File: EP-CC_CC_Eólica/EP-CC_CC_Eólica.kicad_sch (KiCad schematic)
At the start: 19 parts, among them J1 Screw_Terminal_01x03, J2 Screw_Terminal_01x02, Q1 IKW40N120H3, U1 LA100-P, U2 LV25-P

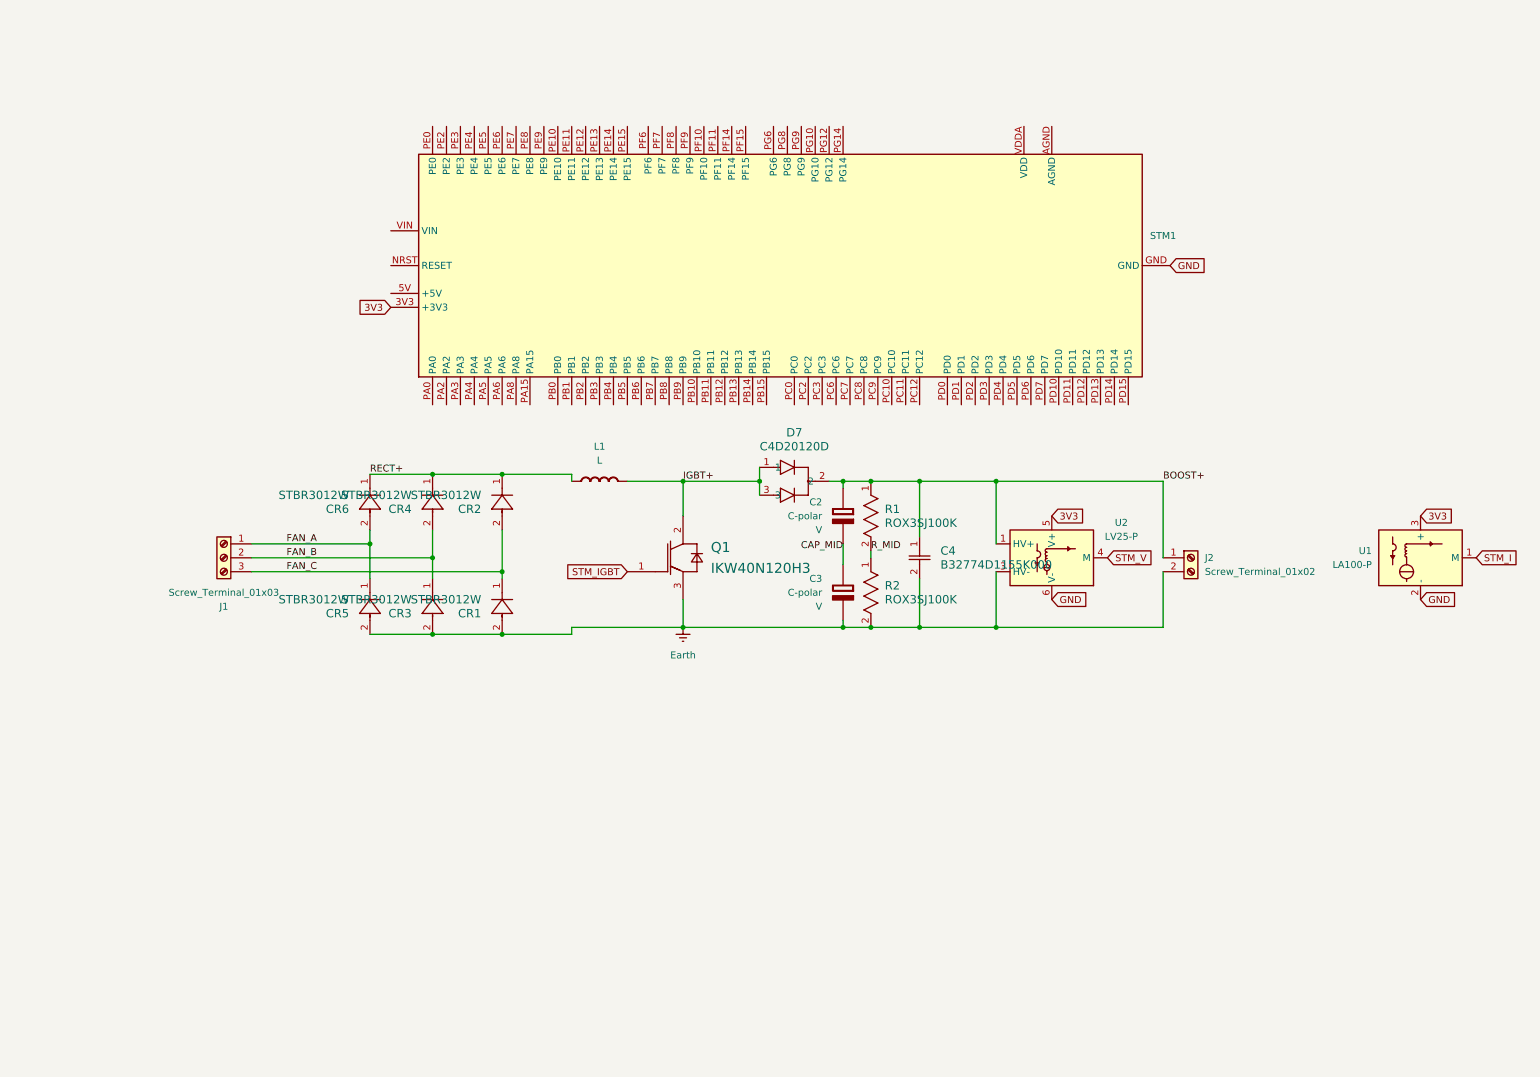
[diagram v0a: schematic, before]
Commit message: 26/10/19
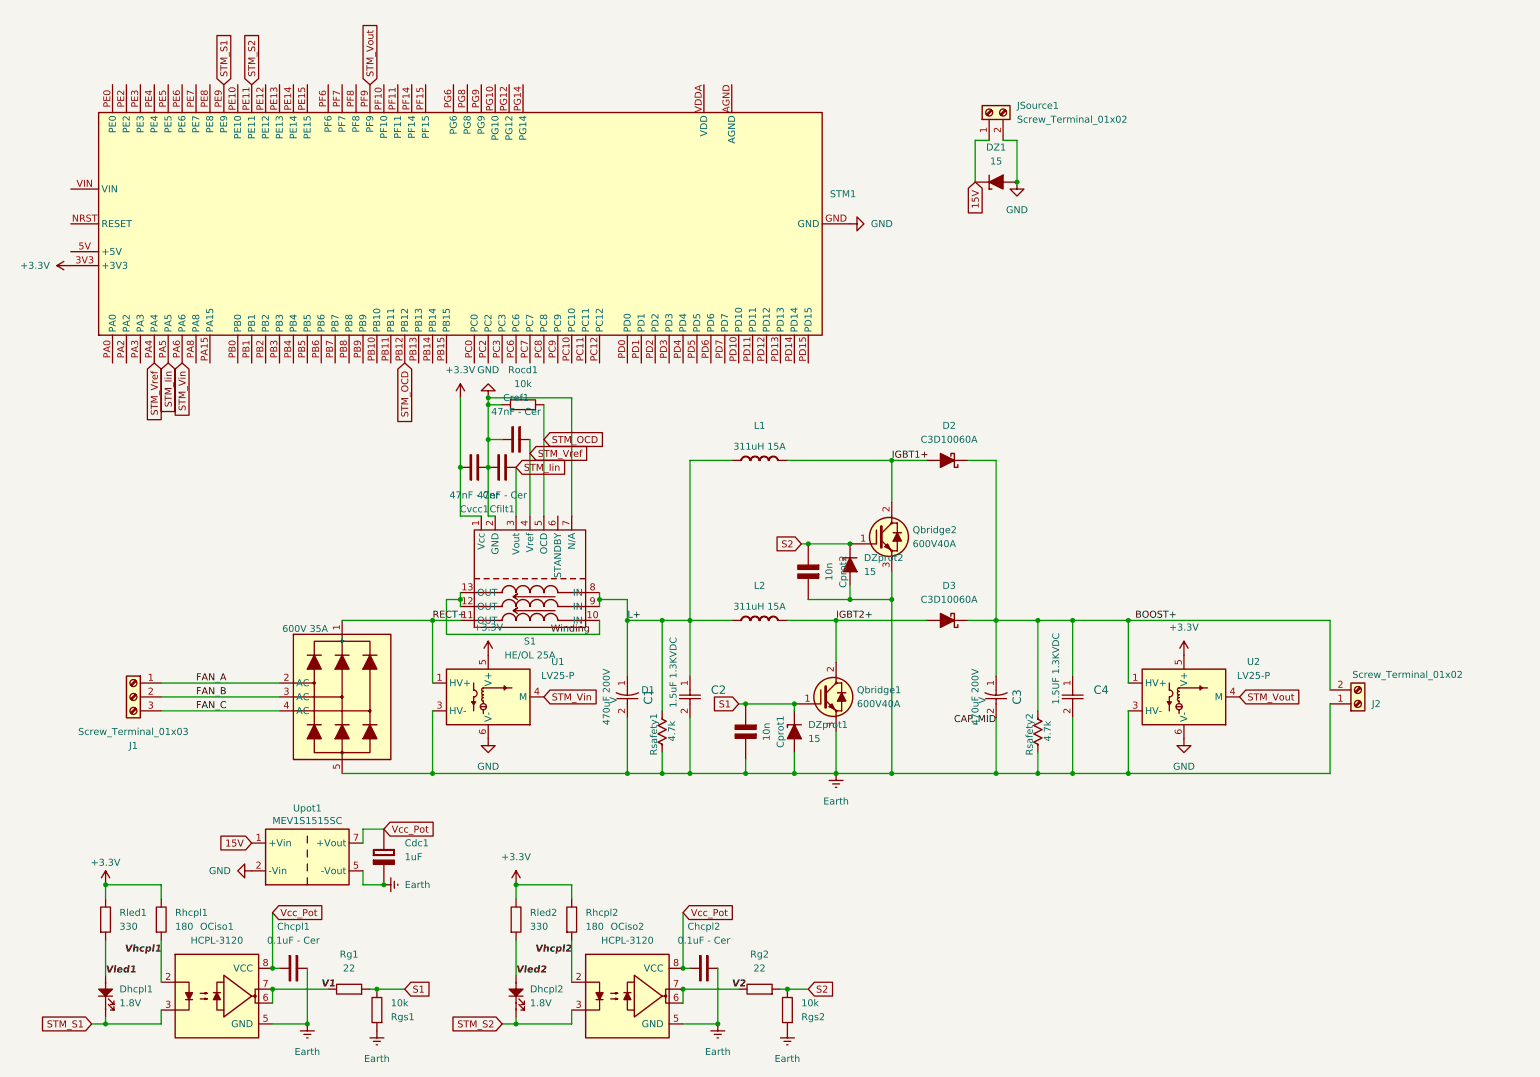
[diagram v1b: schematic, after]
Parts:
- removed C3: C-polar, Capacitor_THT:CP_Radial_D24.0mm_P10.00mm_SnapIn, symbol PCM_Elektuur:C-polar
- removed CR1, CR2, CR3, CR4, CR5, CR6: STBR3012W, Boost:DO-247_STM, symbol Boost:STBR3012W
- removed D7: C4D20120D, Boost:TO-247-3_CRW, symbol Boost:C4D20120D
- removed R1, R2: ROX3SJ100K, Boost:RES_ROX3S_TYCO_TYC, symbol Boost:ROX3SJ100K
- removed U1: LA100-P, Sensor_Current:LEM_LA25-P, symbol Sensor_Current:LA100-P
- added C1: 470uF 200V, Boost:CAP_22 X 35_NCH, symbol Boost:LGU2D471MELZ
- added C2: 1.5uF 1.3KVDC, Boost:CAP_B32774D1155K000_TDK, symbol Boost:B32774D1155K000
- added Cdc1: 1uF, Capacitor_THT:CP_Radial_D5.0mm_P2.00mm, symbol PCM_Elektuur:C-polar
- added Cfilt1, Cref1, Cvcc1: 47nF - Cer, Capacitor_THT:C_Disc_D5.1mm_W3.2mm_P5.00mm, symbol PCM_SL_Devices:Capacitor_NP
- added Chcpl1, Chcpl2: 0.1uF - Cer, Capacitor_THT:C_Disc_D5.1mm_W3.2mm_P5.00mm, symbol PCM_SL_Devices:Capacitor_NP
- added Cprot1, Cprot2: 10n, Capacitor_THT:C_Disc_D6.0mm_W2.5mm_P5.00mm, symbol PCM_Elektuur:C
- added D1: 600V 35A, Boost:VS-36MT160, symbol Boost:VS-36MT160
- added D2, D3: C3D10060A, PCM_Package_TO_SOT_THT_AKL:TO-220-2_Vertical_KA, symbol PCM_Diode_Schottky_AKL:C3D10060A
- added DZ1: 15, Diode_THT:D_DO-27_P5.08mm_Vertical_AnodeUp, symbol PCM_Diode_Zener_AKL:D_Zener_Generic
- added DZprot1, DZprot2: 15, Diode_THT:D_DO-34_SOD68_P10.16mm_Horizontal, symbol PCM_Diode_Zener_AKL:D_Zener_Generic
- added Dhcpl1, Dhcpl2: 1.8V, LED_THT:LED_D5.0mm, symbol PCM_SL_Devices:LED
- added JSource1: Screw_Terminal_01x02, Boost:CONN2_2604-3102_WAG, symbol Connector:Screw_Terminal_01x02
- added L2: 311uH 15A, Boost:SHBC24W-2R1A0311V, symbol PCM_Elektuur:L
- added OCiso1, OCiso2: HCPL-3120, PCM_Package_DIP_AKL:DIP-8_W7.62mm_LongPads, symbol PCM_Optocoupler_Gate_Driver_AKL:HCPL-3120
- added Qbridge2: 600V40A, Boost:TO-220_High, symbol Boost:STGW60V60DF
- added Rg1, Rg2: 22, Resistor_THT:R_Axial_DIN0309_L9.0mm_D3.2mm_P2.54mm_Vertical, symbol PCM_SL_Resistors:Resistor
- added Rgs1, Rgs2, Rocd1: 10k, Resistor_THT:R_Axial_DIN0309_L9.0mm_D3.2mm_P2.54mm_Vertical, symbol PCM_SL_Resistors:Resistor
- added Rhcpl1, Rhcpl2: 180, Resistor_THT:R_Axial_DIN0309_L9.0mm_D3.2mm_P2.54mm_Vertical, symbol PCM_SL_Resistors:Resistor
- added Rled1, Rled2: 330, Resistor_THT:R_Axial_DIN0309_L9.0mm_D3.2mm_P2.54mm_Vertical, symbol PCM_SL_Resistors:Resistor
- added Rsafety1, Rsafety2: 4.7k, Boost:TWM20J4K7E, symbol PCM_Resistor_US_AKL:R_Power_L75.0mm_W9.0mm_P81.28mm
- added S1: HE/OL 25A, Boost:HO 25-N_SP33-1000, symbol Boost:HO_25-NP_SP33-1000
- added U2: LV25-P, Sensor_Voltage:LEM_LV25-P, symbol Sensor_Voltage:LV25-P
- added Upot1: MEV1S1515SC, Library:MEV1S1505SC, symbol Converter_DCDC:MEE1S1515SC
- C3: renamed from C2; value C-polar -> 470uF 200V; footprint Capacitor_THT:CP_Radial_D24.0mm_P10.00mm_SnapIn -> Boost:CAP_22 X 35_NCH; symbol PCM_Elektuur:C-polar -> Boost:LGU2D471MELZ
- C4: value B32774D1155K000 -> 1.5UF 1.3KVDC
- L1: value L -> 311uH 15A; footprint Inductor_THT:L_Axial_L26.0mm_D11.0mm_P7.62mm_Vertical_Fastron_77A -> Boost:SHBC24W-2R1A0311V
- Qbridge1: renamed from Q1; value IKW40N120H3 -> 600V40A; footprint Boost:INF-PG-TO247-3 -> Boost:TO-220_High; symbol Boost:IKW40N120H3 -> Boost:STGW60V60DF; Price (none) -> 1.3386
- renumbered U2 to U1
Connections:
- net CAP_MID is gone; now on net Earth: C3.2
- net STM_V is gone; now on net STM_Vin: U1.4 (M)
- net BOOST+: now also J2.2 (Pin_2), D2.1 (K), D3.1 (K), Rsafety2.1, U2.1 (HV+); no longer J2.1 (Pin_1), U1.1 (HV+)
- net Earth: now also J2.1 (Pin_1), C1.2, C2.2, Cdc1.2 (-), Chcpl1.2, Chcpl2.2, Cprot1.2 (-), Cprot2.2 (-), D1.5 (-), DZprot1.2 (A), DZprot2.2 (A), OCiso1.5 (GND), OCiso2.5 (GND), Qbridge2.3 (E), Rgs1.1, Rgs2.1, Rsafety1.2, Rsafety2.2, U2.3 (HV-), Upot1.5 (-Vout); no longer J2.2 (Pin_2)
- net FAN_A: now also D1.2 (AC)
- net FAN_B: now also D1.3 (AC)
- net FAN_C: now also D1.4 (AC)
- net GND: now also Cfilt1.2, Cref1.2, Cvcc1.1, DZ1.2 (A), JSource1.2 (Pin_2), Rocd1.1, S1.2 (GND), S1.7 (N/A), U2.6 (V-), Upot1.2 (-Vin)
- net RECT+: now also U1.1 (HV+), D1.1 (+), S1.11 (OUT); no longer L1.1 (+)
- net STM_Vref: now reaches STM1.PA4
- net STM_Vref: now also Cref1.1, S1.4 (Vref)
- net STM_Iin: now reaches STM1.PA5
- net STM_Iin: now also Cfilt1.1, S1.3 (Vout)
- net STM_Vin: now reaches STM1.PA6
- net STM_OCD: now reaches STM1.PB12
- net STM_OCD: now also Rocd1.2, S1.5 (OCD)
- net STM_S2: now reaches STM1.PE11
- net STM_S2: now also Dhcpl2.1, OCiso2.3
- net STM_S1: now reaches STM1.PE9
- net STM_S1: now also Dhcpl1.1, OCiso1.3
- net STM_Vout: now reaches STM1.PF9
- net STM_Vout: now also U2.4 (M)
- net 3V3 renamed +3.3V
- net +3.3V: now also Cvcc1.2, Rhcpl1.2, Rhcpl2.2, Rled1.2, Rled2.2, S1.1 (Vcc), U2.5 (V+)
- net IGBT+ renamed IGBT1+
- net IGBT1+: now also D2.2 (A), Qbridge2.2 (C); no longer Qbridge1.2 (COLLECTOR)
- net STM_IGBT renamed S1
- net S1: now also Cprot1.1 (+), DZprot1.1 (K), Rg1.1, Rgs1.2
- new net 15V: DZ1.1 (K), JSource1.1 (Pin_1), Upot1.1 (+Vin)
- new net IGBT2+: D3.2 (A), L2.2 (-), Qbridge1.2 (C)
- new net L+: C1.1, C2.1, L1.1 (+), L2.1 (+), Rsafety1.1, S1.8 (IN), S1.9 (IN)
- new net S2: Cprot2.1 (+), DZprot2.1 (K), Qbridge2.1 (G), Rg2.1, Rgs2.2
- new net V1: OCiso1.6, OCiso1.7, Rg1.2
- new net V2: OCiso2.6, OCiso2.7, Rg2.2
- new net Vcc_Pot: Cdc1.1 (+), Chcpl1.1, Chcpl2.1, OCiso1.8 (VCC), OCiso2.8 (VCC), Upot1.7 (+Vout)
- new net Vhcpl1: OCiso1.2, Rhcpl1.1
- new net Vhcpl2: OCiso2.2, Rhcpl2.1
- new net Vled1: Dhcpl1.2, Rled1.1
- new net Vled2: Dhcpl2.2, Rled2.1
- new net Winding: S1.10 (IN), S1.12 (OUT), S1.13 (OUT)
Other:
- moved on the sheet: C4, J1, J2, STM1, U1
